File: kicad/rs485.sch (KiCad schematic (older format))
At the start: 5 parts, among them J1201 Screw_Terminal_01x05, U1201 ADM2483

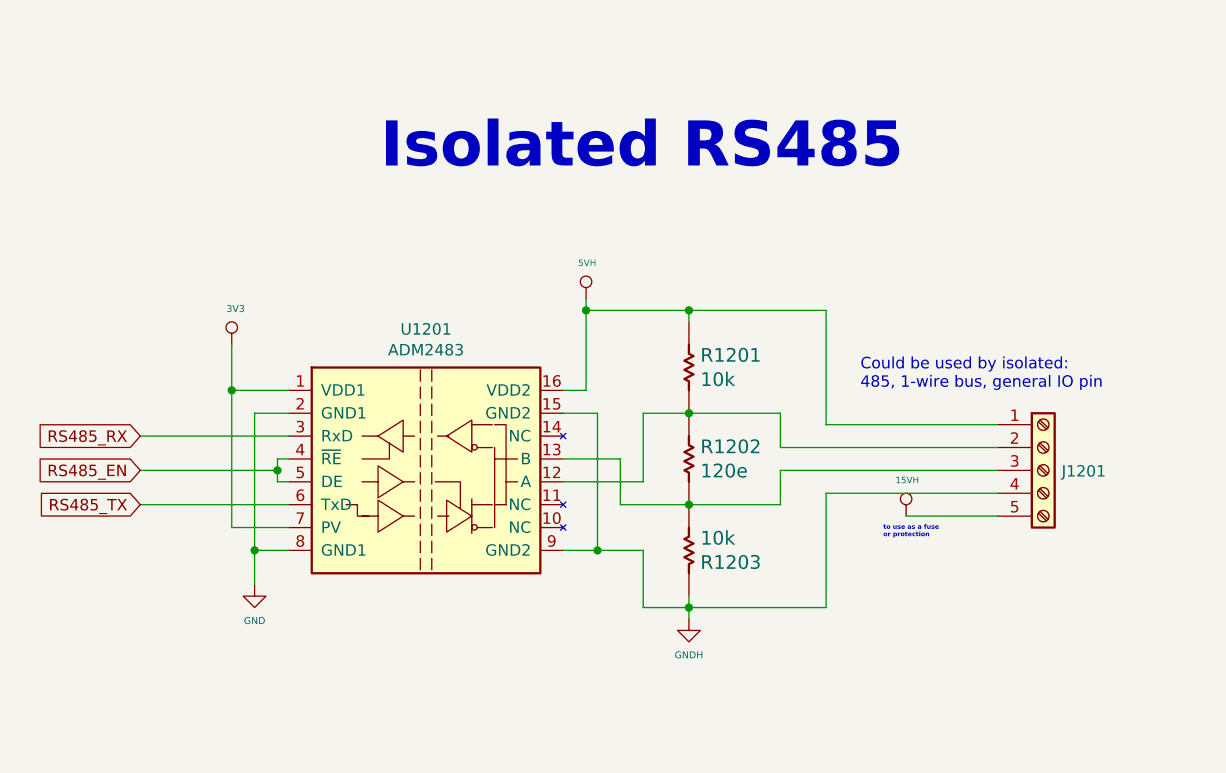
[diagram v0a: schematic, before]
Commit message: begin PCB!! it's amess but IT IS
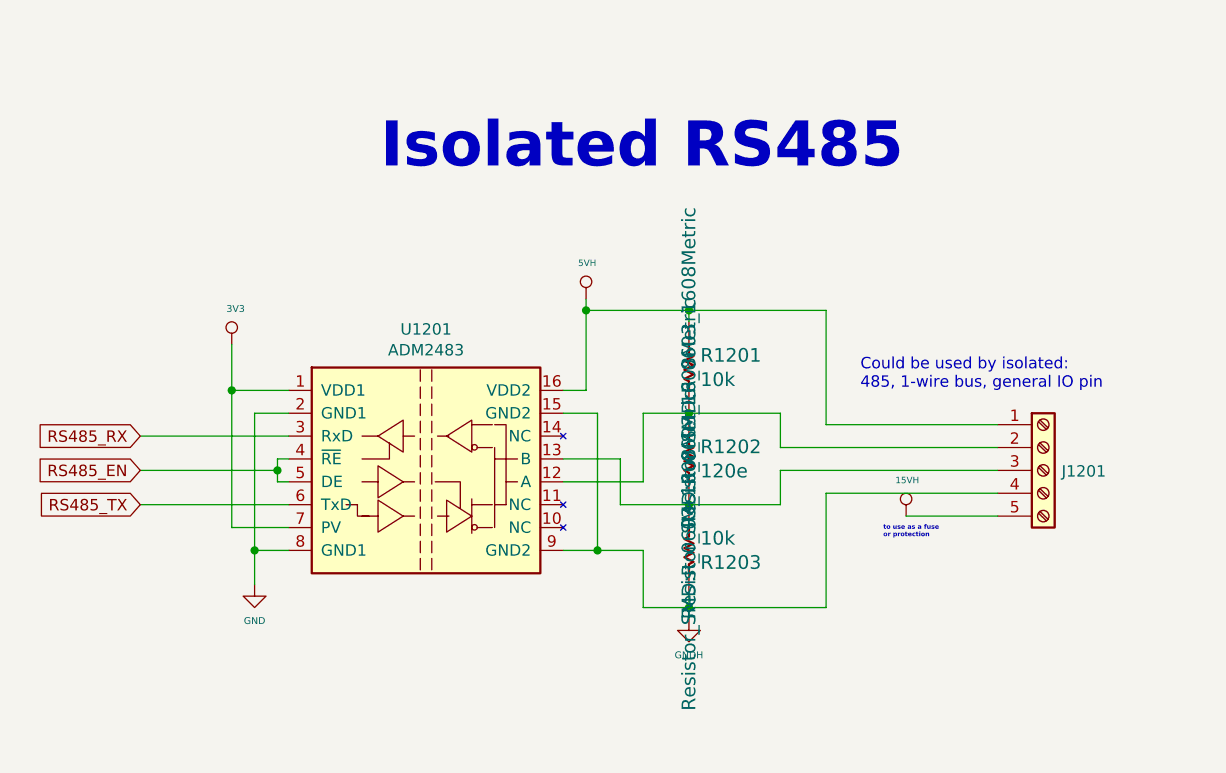
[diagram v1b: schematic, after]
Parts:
- R1201, R1202, R1203: footprint (none) -> Resistor_SMD:R_0603_1608Metric
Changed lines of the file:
@@
 F 0 "R1202" V 5597 2850 60  0000 L CNN
 F 1 "120e" V 5703 2850 60  0000 L CNN
-F 2 "" H 5650 2800 60  0000 C CNN
+F 2 "Resistor_SMD:R_0603_1608Metric" H 5650 2800 60  0000 C CNN
 F 3 "" H 5650 2800 60  0000 C CNN
 	1    5650 2800
@@
 F 0 "R1203" V 5597 3250 60  0000 L CNN
 F 1 "10k" V 5703 3250 60  0000 L CNN
-F 2 "" H 5650 3200 60  0000 C CNN
+F 2 "Resistor_SMD:R_0603_1608Metric" H 5650 3200 60  0000 C CNN
 F 3 "" H 5650 3200 60  0000 C CNN
 	1    5650 3200
@@
 F 0 "R1201" V 5597 2450 60  0000 L CNN
 F 1 "10k" V 5703 2450 60  0000 L CNN
-F 2 "" H 5650 2400 60  0000 C CNN
+F 2 "Resistor_SMD:R_0603_1608Metric" H 5650 2400 60  0000 C CNN
 F 3 "" H 5650 2400 60  0000 C CNN
 	1    5650 2400

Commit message: I've passed all footprin to layout BUT...
I've passed all, first glance... I need to confirm in details a lot of
things. The objetive for these is to have an aproximation of the size
I'll need to make the board.. then I choose the final detailed footprint
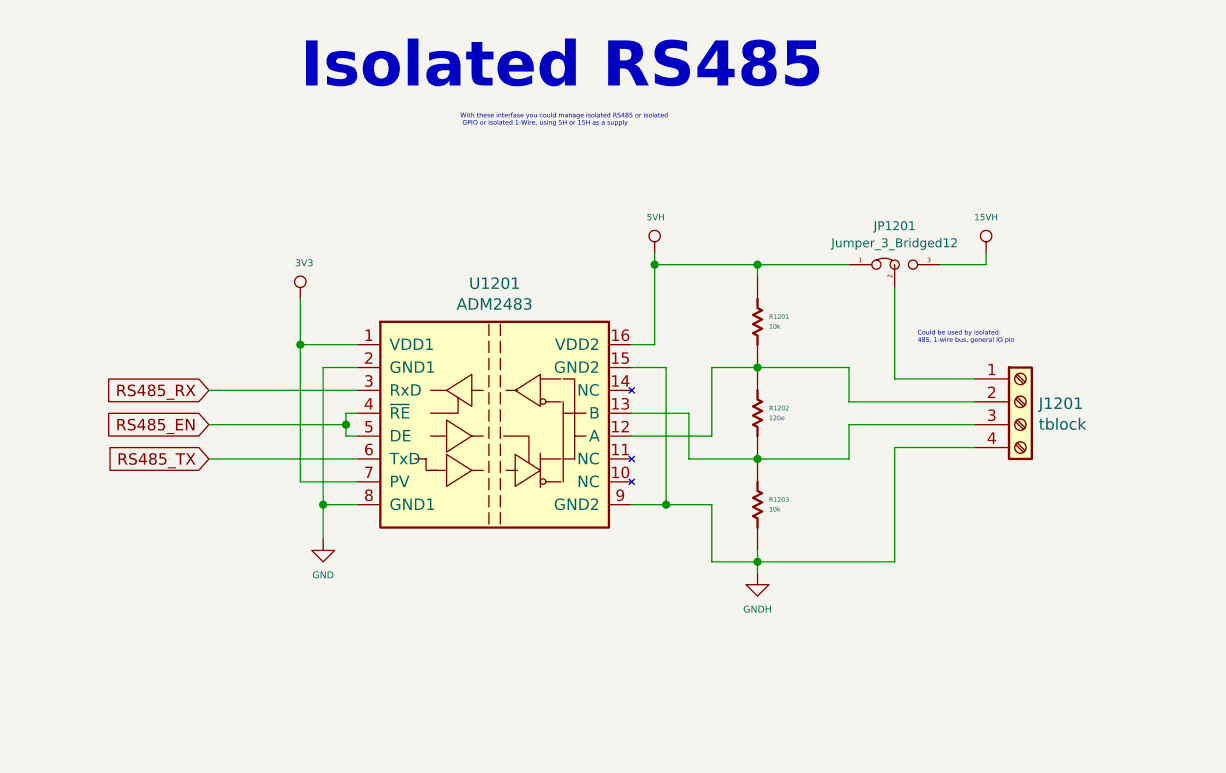
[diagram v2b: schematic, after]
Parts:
- removed J1201: Screw_Terminal_01x05, symbol Connector:Screw_Terminal_01x05
- added J1201: tblock, TerminalBlock_RND:TerminalBlock_RND_205-00289_1x04_P5.08mm_Horizontal, symbol Connector:Screw_Terminal_01x04
- added JP1201: Jumper_3_Bridged12, Jumper:SolderJumper-3_P1.3mm_Open_RoundedPad1.0x1.5mm, symbol servo:Jumper_3_Bridged12
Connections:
- net 15VH: now also JP1201.3 (B)
- net 5VH: now also JP1201.1 (A)
- net GNDH: now also R1203.2, J1201.4 (Pin_4); no longer R1203.1
- net at R1201.2, R1202.1, U1201.12 (A): now also J1201.2 (Pin_2)
- net at R1202.2, U1201.13 (B): now also R1203.1, J1201.3 (Pin_3); no longer R1203.2
- new net: J1201.1 (Pin_1), JP1201.2 (C)
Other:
- note added: "With these interfase you could manage isolated RS485 or isolated \n GPIO or isolated 1-Wire, using 5H or 15H as a supply"
- note removed: "to use as a fuse \nor protection"
- moved on the sheet: R1201, R1202, R1203, U1201
